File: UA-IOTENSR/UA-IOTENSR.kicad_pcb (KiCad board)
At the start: 4 copper layers, 95.2 x 79 mm, 37 parts, among them IC1 BQ2000TPN-B5, J1 Conn_01x04_Male, J2 ZX62-AB-5PA_31_, SW1 SW_Push, U1 ESP32-S3-MINI-1, U2 AP63203WU

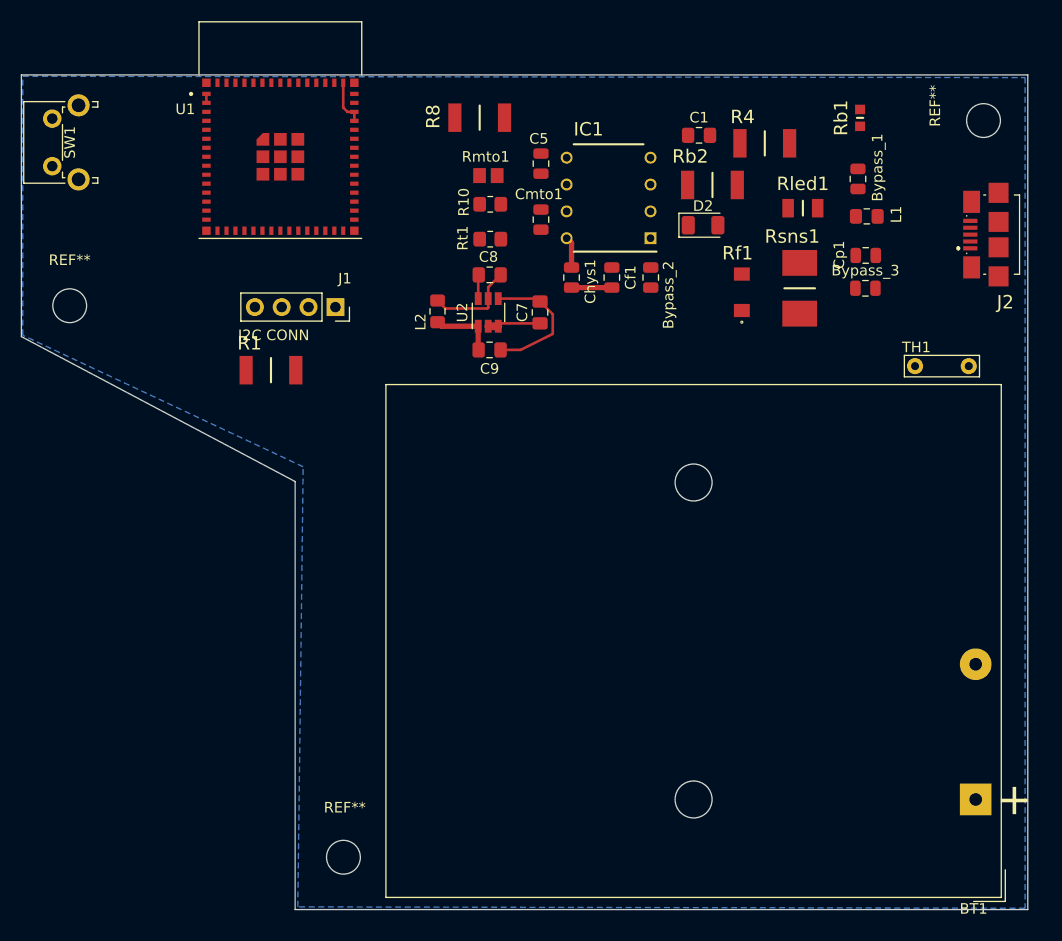
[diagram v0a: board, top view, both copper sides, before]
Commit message: pushbutton, esp antenna, condensing, title + james!!
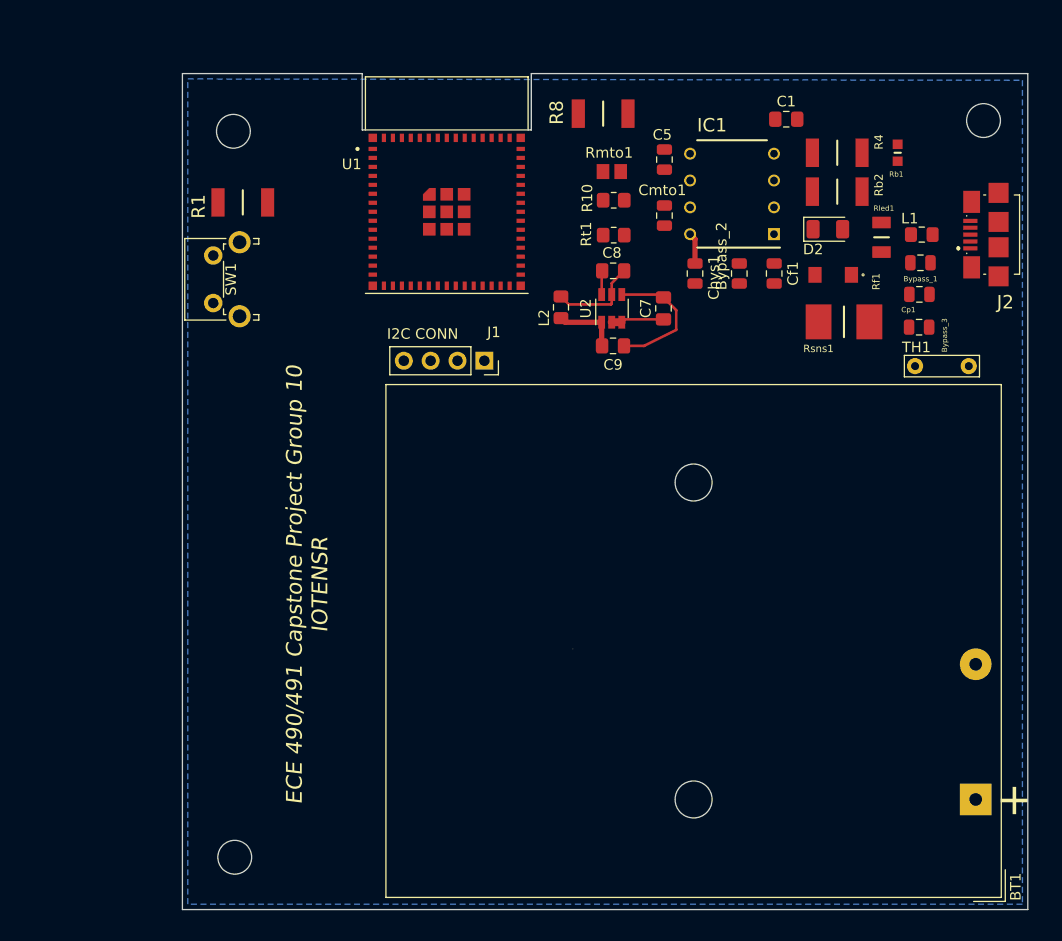
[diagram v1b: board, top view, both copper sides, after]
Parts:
- removed the REF** at (111.3, 77.5)
- removed the REF** at (137.2, 129.7)
- added G***: LOGO, SamacSys_Parts:negative_cropped_james, F.Cu at (149.4, 110.2)
- added REF**: MountingHole_3.2mm_M3, MountingHole:MountingHole_3.2mm_M3, F.Cu at (126.7, 61.0)
- added REF**: MountingHole_3.2mm_M3, MountingHole:MountingHole_3.2mm_M3, F.Cu at (126.9, 129.7)
- moved SW1 20.0 mm to (124.8, 77.2)
- moved U1 16.6 mm to (146.9, 68.6)
- moved R1 16.1 mm to (127.6, 67.7)
- moved Cf1 15.4 mm to (177.9, 74.4)
- moved J1 15.0 mm to (150.5, 82.7)
- moved Rb2 11.8 mm to (183.9, 66.7)
- moved D2 11.8 mm to (183.0, 70.2)
- moved C7 11.7 mm to (167.4, 77.7)
- moved C8 11.7 mm to (162.7, 74.2)
- moved C5 11.7 mm to (167.5, 63.6)
- moved C9 11.7 mm to (162.7, 81.3)
- moved Chys1 11.7 mm to (170.4, 74.4)
- moved Cmto1 11.7 mm to (167.5, 68.9)
- moved IC1 11.7 mm to (173.9, 66.9)
- moved L2 11.7 mm to (157.7, 77.6)
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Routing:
- net BAT-: track 18.2 -> 12.9 mm
- net Net-(Cf1-Pad1): track 3.81 -> 0.00 mm
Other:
- board size 95.2 x 79 mm -> 80 x 79.1 mm
- board text added: "ECE 490/491 Capstone Project Group 10 IOTENSR"
